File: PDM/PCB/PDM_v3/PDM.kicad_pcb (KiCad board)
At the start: 4 copper layers, 65 x 80 mm, 59 parts, among them IC1 SN74LVC1GU04DBVT, J1 12V BAT, J10 RASPBERRY PI, J11 EMU, J12 Conn_01x02_Male, J13 SAFETY SYSTEM, J16 GND, J2 EMU PIN 21 GN(AUX1), J3 EMU PIN 13 GN (AUX2), J4 BACK LIGHT, J5 COILS, J6 INJECTORS, J7 LSU 4.9, J8 RACE TCS, J9 STM BOX, U1 BTS50010-1TAE, U2 BTS50010-1TAE, U3 BTS50010-1TAE, U4 LM2937xMP

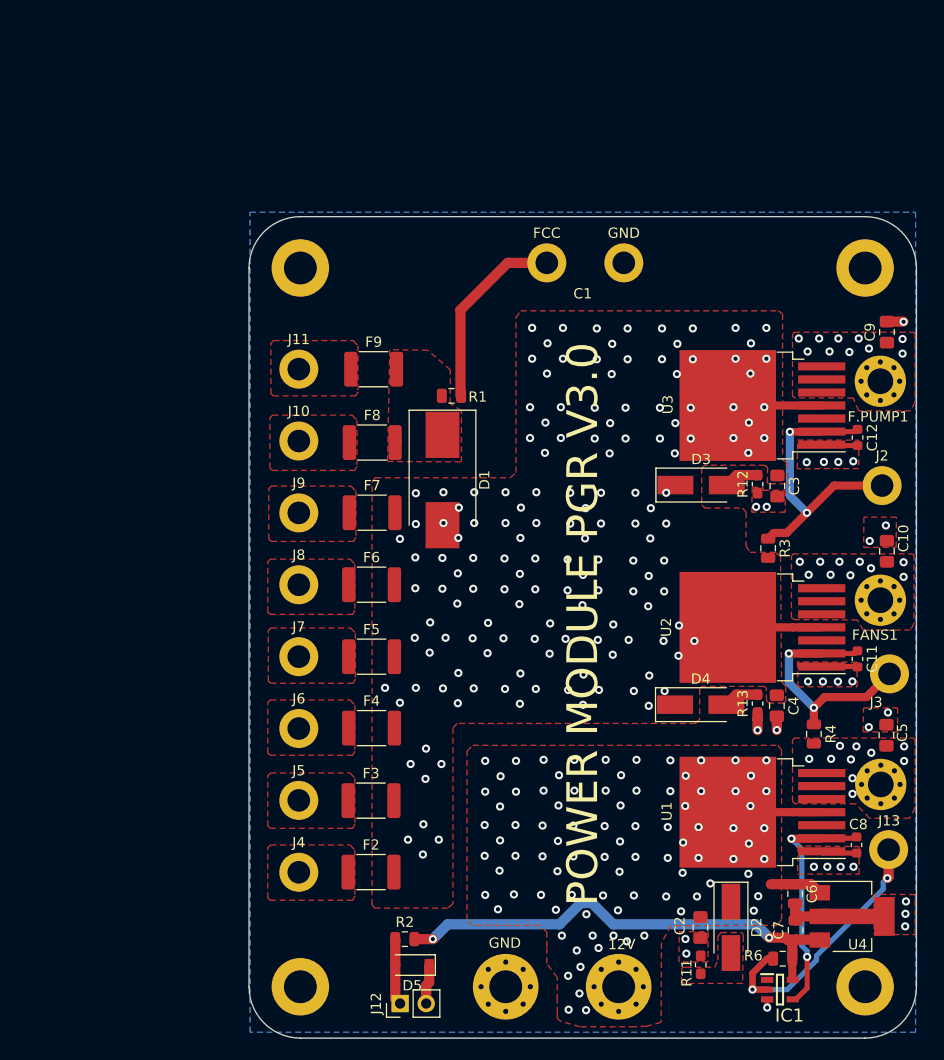
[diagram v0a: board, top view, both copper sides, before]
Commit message: Update PDM PCB
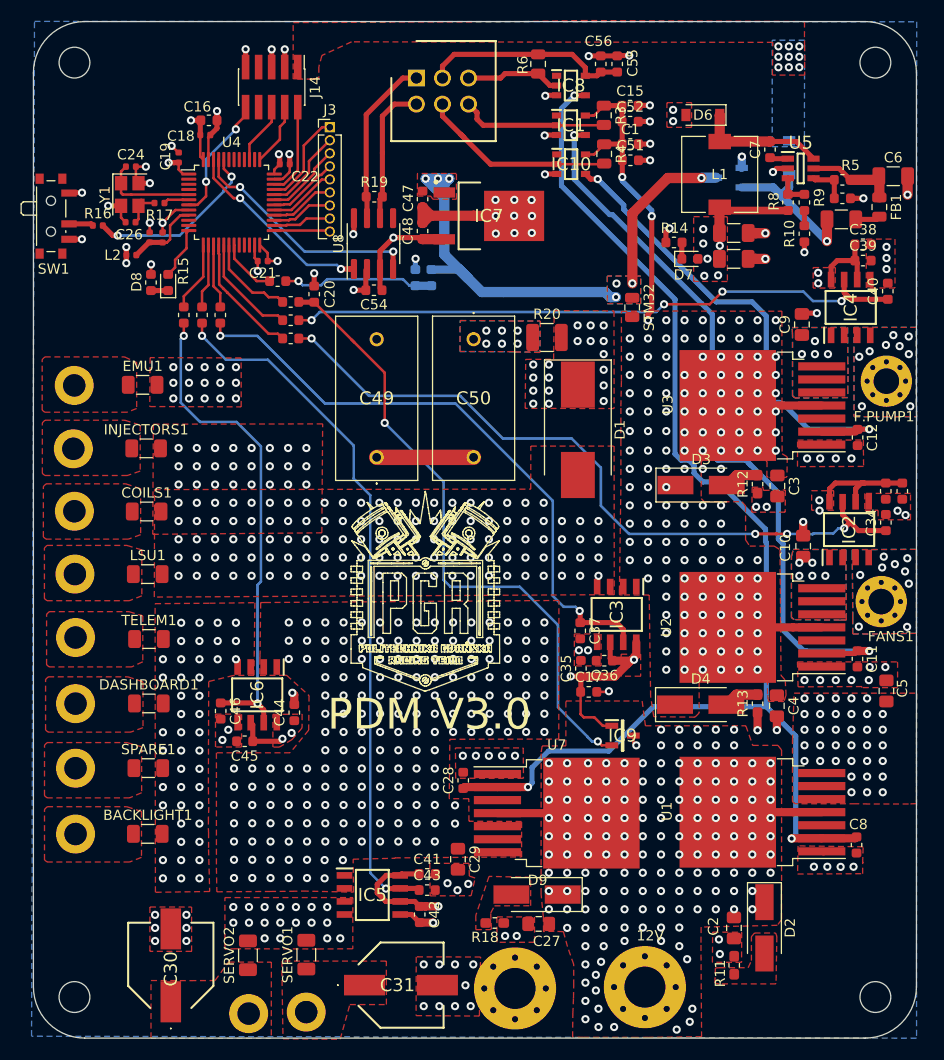
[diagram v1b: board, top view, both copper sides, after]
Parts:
- removed 12V1: 85 K1 (starter), MountingHole:MountingHole_2.5mm_Pad_Via
- removed D5: D_Schottky, Diode_SMD:D_SOD-123
- removed J12: Conn_01x02_Male, Connector_PinHeader_2.54mm:PinHeader_1x02_P2.54mm_Vertical
- removed J13: SAFETY SYSTEM, MountingHole:MountingHole_2.2mm_M2_DIN965_Pad
- added C13: 10uF, Capacitor_SMD:C_1206_3216Metric, F.Cu at (142.2, 44.6)
- added C14: 10uF, Capacitor_SMD:C_1206_3216Metric, F.Cu at (142.2, 47.1)
- added C15: 0.1uF, Capacitor_SMD:C_0603_1608Metric, F.Cu at (132.1, 32.2)
- added C16: 4u7, Capacitor_SMD:C_0603_1608Metric, F.Cu at (91.1, 33.6)
- added C17: 0.1uF, Capacitor_SMD:C_0603_1608Metric, F.Cu at (128.1, 89.3)
- added C18: 100n, Capacitor_SMD:C_0402_1005Metric, F.Cu at (90.7, 35.1)
- added C19: 100n, Capacitor_SMD:C_0402_1005Metric, F.Cu at (88.1, 37.2)
- added C20: 0.1uF, Capacitor_SMD:C_0603_1608Metric, F.Cu at (101.3, 50.5)
- added C21: 100n, Capacitor_SMD:C_0402_1005Metric, F.Cu at (96.3, 47.3)
- added C22: 100n, Capacitor_SMD:C_0402_1005Metric, F.Cu at (98.5, 37.9)
- added C23: 1u, Capacitor_SMD:C_0402_1005Metric, F.Cu at (85.3, 45.0)
- added C24: 12p, Capacitor_SMD:C_0402_1005Metric, F.Cu at (83.5, 38.1)
- added C25: 10n, Capacitor_SMD:C_0402_1005Metric, F.Cu at (86.6, 45.0)
- added C26: 12p, Capacitor_SMD:C_0402_1005Metric, F.Cu at (83.5, 43.5)
- added C27: 100nF, Capacitor_SMD:C_0805_2012Metric_Pad1.15x1.40mm_HandSolder, F.Cu at (123.2, 111.9)
- added C28: 150nF, Capacitor_SMD:C_0603_1608Metric, F.Cu at (115.9, 97.9)
- added C29: 10nF, Capacitor_SMD:C_0805_2012Metric_Pad1.15x1.40mm_HandSolder, F.Cu at (115.3, 105.6)
- added C30: 100uF, EEETP1C101AP:EEE0JA471UAP, F.Cu at (87.4, 115.9)
- added C31: 100uF, EEETP1C101AP:EEE0JA471UAP, F.Cu at (109.8, 117.8)
- added C32: 47nF, Capacitor_SMD:C_0603_1608Metric, F.Cu at (157.0, 69.7)
- added C33: 47nF, Capacitor_SMD:C_0603_1608Metric, F.Cu at (158.6, 69.7)
- added C34: 4.7nF, Capacitor_SMD:C_0603_1608Metric, F.Cu at (157.0, 72.8)
- added C35: 47nF, Capacitor_SMD:C_0603_1608Metric, F.Cu at (127.3, 87.0)
- added C36: 47nF, Capacitor_SMD:C_0603_1608Metric, F.Cu at (129.6, 86.2)
- added C37: 4.7nF, Capacitor_SMD:C_0603_1608Metric, F.Cu at (127.3, 83.3)
- added C38: 47nF, Capacitor_SMD:C_0603_1608Metric, F.Cu at (154.8, 45.7)
- added C39: 47nF, Capacitor_SMD:C_0603_1608Metric, F.Cu at (154.8, 47.3)
- added C40: 4.7nF, Capacitor_SMD:C_0603_1608Metric, F.Cu at (157.2, 50.3)
- added C41: 47nF, Capacitor_SMD:C_0603_1608Metric, F.Cu at (112.4, 107.0)
- added C42: 47nF, Capacitor_SMD:C_0603_1608Metric, F.Cu at (111.6, 111.0)
- added C43: 4.7nF, Capacitor_SMD:C_0603_1608Metric, F.Cu at (112.4, 108.6)
- added C44: 47nF, Capacitor_SMD:C_0603_1608Metric, F.Cu at (99.4, 91.3)
- added C45: 47nF, Capacitor_SMD:C_0603_1608Metric, F.Cu at (94.6, 94.1)
- added C46: 4.7nF, Capacitor_SMD:C_0603_1608Metric, F.Cu at (92.2, 91.1)
- added C47: 0.47uF, Capacitor_SMD:C_0603_1608Metric, F.Cu at (111.9, 41.3)
- added C48: 22uF, Capacitor_SMD:C_0603_1608Metric, F.Cu at (111.9, 44.4)
- added C49: SCMR18H105PRBB0, SCMR18H105PRBB0:SCMR18H105PRBB0, F.Cu at (107.4, 66.4)
- added C50: SCMR18H105PRBB0, SCMR18H105PRBB0:SCMR18H105PRBB0, F.Cu at (116.9, 54.9)
- added C51: 1uF, Capacitor_SMD:C_0603_1608Metric, F.Cu at (132.1, 37.5)
- added C52: 1uF, Capacitor_SMD:C_0603_1608Metric, F.Cu at (132.1, 33.8)
- added C54: 0.47uF, Capacitor_SMD:C_0603_1608Metric, F.Cu at (107.2, 50.2)
- added C55: 0.1uF, Capacitor_SMD:C_0603_1608Metric, F.Cu at (130.9, 28.1)
- added C56: 1uF, Capacitor_SMD:C_0603_1608Metric, F.Cu at (129.3, 28.1)
- added D11: B5819W, Diode_SMD:D_SOD-123, B.Cu at (147.6, 37.3)
- added D6: B5819W, Diode_SMD:D_SOD-123, F.Cu at (139.2, 33.1)
- added D7: LED, LED_SMD:LED_0603_1608Metric, F.Cu at (137.9, 47.1)
- added D8: BLUE, LED_SMD:LED_0603_1608Metric, F.Cu at (87.1, 49.4)
- added D9: D_TVS_ALT, Diode_SMD:D_SMA_Handsoldering, F.Cu at (123.0, 109.0)
- added F1: Polyfuse_Small, Fuse:Fuse_1206_3216Metric, F.Cu at (152.7, 43.3)
- added FB1: 600 @ 600Mhz, Inductor_SMD:L_0805_2012Metric, F.Cu at (156.4, 42.1)
- added IC10: BU4S584G2-TR, BU4S584G2-TR:SOT95P280X125-5N, F.Cu at (126.4, 37.9)
- added IC2: MLX91221KDC-ABR-020-SP, MLX91221KDC-ABR-020-SP:SOIC127P600X173-8N, F.Cu at (153.4, 73.5)
- added IC3: MLX91221KDC-ABR-020-SP, MLX91221KDC-ABR-020-SP:SOIC127P600X173-8N, F.Cu at (130.8, 81.7)
- added IC4: MLX91221KDC-ABR-020-SP, MLX91221KDC-ABR-020-SP:SOIC127P600X173-8N, F.Cu at (153.6, 51.8)
- added IC5: MLX91221KDC-ABR-020-SP, MLX91221KDC-ABR-020-SP:SOIC127P600X173-8N, F.Cu at (107.0, 109.1)
- added IC6: MLX91221KDC-ABR-020-SP, MLX91221KDC-ABR-020-SP:SOIC127P600X173-8N, F.Cu at (95.8, 89.6)
- added IC7: KF50BDT-TR, KF50BDT-TR:TO228P972X240-3N, F.Cu at (118.4, 42.9)
- added IC8: BU4S584G2-TR, BU4S584G2-TR:SOT95P280X125-5N, F.Cu at (126.4, 30.2)
- added IC9: TMP236A4DBZT, TMP236A4DBZT:SOT95P237X112-3N, F.Cu at (131.4, 93.5)
- added J14: SWD, Connector_PinHeader_1.27mm:PinHeader_2x05_P1.27mm_Vertical_SMD, F.Cu at (97.2, 30.4)
- added J15: SERVO_GEAR, MountingHole:MountingHole_2.2mm_M2_DIN965_Pad, F.Cu at (100.6, 120.5)
- added J17: SERVO_CLUTCH, MountingHole:MountingHole_2.2mm_M2_DIN965_Pad, F.Cu at (95.0, 120.6)
- added L1: 10uH, Inductor_SMD:L_7.3x7.3_H4.5, F.Cu at (140.8, 38.9)
- added L2: 39n, Inductor_SMD:L_0402_1005Metric, F.Cu at (83.5, 46.7)
- added Q1: AO3401A, AO3401A:SOT95P280X125-3N, B.Cu at (141.7, 39.2)
- added R10: 270, Resistor_SMD:R_0603_1608Metric, F.Cu at (149.1, 44.7)
- added R14: 1k, Resistor_SMD:R_0603_1608Metric, F.Cu at (136.4, 45.5)
- added R15: 1k5, Resistor_SMD:R_0603_1608Metric, F.Cu at (85.4, 49.4)
- added R16: 10k, Resistor_SMD:R_0402_1005Metric, F.Cu at (80.3, 43.9)
- added R17: 47, Resistor_SMD:R_0402_1005Metric, F.Cu at (86.3, 41.7)
- added R18: 1R, Resistor_SMD:R_0603_1608Metric_Pad1.05x0.95mm_HandSolder, F.Cu at (118.9, 111.8)
- added R19: R_Small, Resistor_SMD:R_0603_1608Metric, F.Cu at (107.2, 41.1)
- added R20: R_Small, Resistor_SMD:R_1210_3225Metric, F.Cu at (124.0, 54.8)
- added R21: 6.8k, Resistor_SMD:R_0603_1608Metric, B.Cu at (111.2, 48.9)
- added R22: 0, Resistor_SMD:R_0603_1608Metric, F.Cu at (90.4, 52.6)
- added R23: 0, Resistor_SMD:R_0603_1608Metric, F.Cu at (92.2, 52.6)
- added R24: 0, Resistor_SMD:R_0603_1608Metric, F.Cu at (99.1, 54.9)
- added R25: 0, Resistor_SMD:R_0603_1608Metric, F.Cu at (99.1, 53.1)
- added R26: 0, Resistor_SMD:R_0603_1608Metric, F.Cu at (99.1, 51.3)
- added R27: 0, Resistor_SMD:R_0603_1608Metric, F.Cu at (97.8, 49.3)
- added R5: 100k, Resistor_SMD:R_0603_1608Metric, F.Cu at (152.8, 39.4)
- added R7: 68k, Resistor_SMD:R_0603_1608Metric, F.Cu at (152.8, 41.2)
- added R8: 47k, Resistor_SMD:R_0603_1608Metric, F.Cu at (147.5, 41.6)
- added R9: 15k, Resistor_SMD:R_0603_1608Metric, F.Cu at (149.1, 41.6)
- added SERVO1: 15, Fuse:Fuse_1206_3216Metric, F.Cu at (100.6, 114.9)
- added SERVO2: 15, Fuse:Fuse_1206_3216Metric, F.Cu at (94.9, 114.9)
- added STM32: 2, Fuse:Fuse_0805_2012Metric, F.Cu at (132.3, 51.8)
- added SW1: SW_SPDT, Button_Switch_SMD:SW_SPDT_PCM12, F.Cu at (76.0, 43.0)
- added U5: MP2359, MP2359DT-LF-P:SOT95P280X145-6N, F.Cu at (148.7, 38.3)
- added U7: BTS50010-1TAE, Package_TO_SOT_SMD:TO-263-7_TabPin4, F.Cu at (125.0, 101.1)
- added U8: MCP2561-E-SN, Package_SO:SOIC-8_3.9x4.9mm_P1.27mm, F.Cu at (107.1, 45.6)
- added Y1: 8MHz, Crystal:Crystal_SMD_3225-4Pin_3.2x2.5mm, F.Cu at (83.4, 40.8)
- BACKLIGHT1: renamed from F2; footprint Fuse:Fuse_1812_4532Metric_Pad1.30x3.40mm_HandSolder -> Fuse:Fuse_1206_3216Metric
- C1: value 0.2F -> 0.1uF; footprint Kondensator:Kondensator -> Capacitor_SMD:C_0603_1608Metric
- C6: value 0.1uF -> 10uF; footprint Capacitor_SMD:C_0805_2012Metric -> Capacitor_SMD:C_1206_3216Metric
- C7: value 10uF -> 10nF; footprint Capacitor_SMD:C_0805_2012Metric -> Capacitor_SMD:C_0603_1608Metric
- COILS1: renamed from F3; footprint Fuse:Fuse_1812_4532Metric_Pad1.30x3.40mm_HandSolder -> Fuse:Fuse_1206_3216Metric
- DASHBOARD1: renamed from F7; footprint Fuse:Fuse_1812_4532Metric_Pad1.30x3.40mm_HandSolder -> Fuse:Fuse_1206_3216Metric
- EMU1: renamed from F9; footprint Fuse:Fuse_1812_4532Metric_Pad1.30x3.40mm_HandSolder -> Fuse:Fuse_1206_3216Metric
- H1, H2, H3, H4: footprint MountingHole:MountingHole_3.2mm_M3_DIN965_Pad -> MountingHole:MountingHole_3mm
- IC1: value SN74LVC1GU04DBVT -> BU4S584G2-TR; footprint SN74LVC1GU04DBVT:SOT95P280X145-5N -> BU4S584G2-TR:SOT95P280X125-5N
- INJECTORS1: renamed from F4; footprint Fuse:Fuse_1812_4532Metric_Pad1.30x3.40mm_HandSolder -> Fuse:Fuse_1206_3216Metric
- J1, J16: footprint MountingHole:MountingHole_3.2mm_M3_Pad_Via -> MountingHole:MountingHole_4mm_Pad_Via
- J10: value RASPBERRY PI -> TELEM
- J2: value EMU PIN 21 GN(AUX1) -> 90130-1106; footprint MountingHole:MountingHole_2.2mm_M2_DIN965_Pad -> 90130-1106:SHDR6W65P254_2X3_996X975X1110P
- J3: value EMU PIN 13 GN (AUX2) -> Conn_01x09_Male; footprint MountingHole:MountingHole_2.2mm_M2_DIN965_Pad -> Connector_PinHeader_1.27mm:PinHeader_1x09_P1.27mm_Vertical
- J4: value BACK LIGHT -> BACKLIGHT
- J9: value STM BOX -> DASHBOARD
- LSU1: renamed from F5; footprint Fuse:Fuse_1812_4532Metric_Pad1.30x3.40mm_HandSolder -> Fuse:Fuse_1206_3216Metric
- R1: value 0.1 -> 22k; footprint Resistor_SMD:R_0805_2012Metric -> Resistor_SMD:R_0603_1608Metric; moved to B.Cu
- R2: value 100 -> 0; footprint Resistor_SMD:R_0805_2012Metric -> Resistor_SMD:R_0603_1608Metric
- R3, R4: value 10k -> 100k
- R6: value 100 -> 100k
- SPARE1: renamed from F6; footprint Fuse:Fuse_1812_4532Metric_Pad1.30x3.40mm_HandSolder -> Fuse:Fuse_1206_3216Metric
- TELEM1: renamed from F8; footprint Fuse:Fuse_1812_4532Metric_Pad1.30x3.40mm_HandSolder -> Fuse:Fuse_1206_3216Metric
- U4: value LM2937xMP -> STM32F103C8Tx; footprint Package_TO_SOT_SMD:SOT-223-3_TabPin2 -> Package_QFP:LQFP-48_7x7mm_P0.5mm
- moved U4 92.1 mm to (93.3, 41.6)
- moved R6 90.3 mm to (123.2, 28.1), turned to 270 degrees
- moved IC1 86.6 mm to (126.3, 34.1)
- moved J3 76.2 mm to (102.9, 34.3)
- moved C7 76.1 mm to (145.7, 36.5)
- moved C6 70.5 mm to (157.7, 39.1), turned to 0 degrees
- moved R2 64.5 mm to (88.6, 52.6), turned to 90 degrees
- moved J2 60.3 mm to (111.3, 29.5)
- moved R4 60.1 mm to (129.6, 36.9)
- moved R3 45.1 mm to (129.6, 33.1)
- moved COILS1 35.6 mm to (85.0, 71.7)
- moved J5 35.6 mm to (78.0, 71.7)
- moved INJECTORS1 35.0 mm to (85.0, 65.6)
- moved J6 35.0 mm to (77.9, 65.6)
- moved H1 29.7 mm to (78.0, 28.0)
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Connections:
- BACKLIGHT1 pad 2: 12V_OUT1 -> 12V_SYSTEMS_OUT
- C1 pad 1: Net-(C1-Pad1) -> 12V_MAIN_IN
- C10 pad 1: Net-(C10-Pad1) -> FANS_MOS_IN
- C11 pad 1: IN_2 -> IN_FAN
- C12 pad 1: IN_3 -> IN_FUEL
- C3 pad 1: 12V_OUT1 -> 12V_MAIN_IN
- C4 pad 1: 12V_OUT1 -> 12V_MAIN_IN
- C5 pad 1: 12V_OUT1 -> 12V_MAIN_IN
- C6 pad 1: 12V_BAT -> BUCK_IN
- C7 pad 1: +3V3 -> BUCK_BST
- C7 pad 2: GND -> BUCK_SW
- C8 pad 1: IN_1 -> IN_MAIN_12V
- C9 pad 1: Net-(C9-Pad1) -> FUEL_MOS_IN
- COILS1 pad 2: 12V_OUT1 -> 12V_MAIN_OUT
- D1 pad 2: 12V_OUT1 -> 12V_MAIN_OUT
- D3 pad 1: 12V_OUT1 -> 12V_MAIN_IN
- D4 pad 1: 12V_OUT1 -> 12V_MAIN_IN
- DASHBOARD1 pad 2: 12V_OUT1 -> 12V_SYSTEMS_OUT
- F.PUMP1 pad 1: Net-(C9-Pad1) -> FUEL_MOS_OUT
- FANS1 pad 1: Net-(C10-Pad1) -> FANS_MOS_OUT
- IC1 pad 2: Net-(IC1-Pad2) -> EMU_AUX2
- IC1 pad 4: IN_1 -> IN_FAN
- IC1 pad 5: +3V3 -> 12V_MAIN_IN
- INJECTORS1 pad 2: 12V_OUT1 -> 12V_MAIN_OUT
- J2 pad 1: IN_3 -> CAN_H
- J3 pad 1: IN_2 -> /STM32F103C8T6/PA12
- LSU1 pad 2: 12V_OUT1 -> 12V_MAIN_OUT
- R1 pad 1: Net-(D1-Pad1) -> VOLTAGE_SENS
- R1 pad 2: Net-(C1-Pad1) -> 12V_STM32
- R2 pad 1: BSPD_IN -> CURRENT_12V_SYSTEMS
- R2 pad 2: +3V3 -> /STM32F103C8T6/PA3
- R3 pad 1: IN_3 -> 12V_MAIN_IN
- R3 pad 2: 12V_OUT1 -> EMU_AUX2
- R4 pad 1: IN_2 -> 12V_MAIN_IN
- R4 pad 2: 12V_OUT1 -> EMU_AUX1
- R6 pad 1: +3V3 -> 12V_BAT
- R6 pad 2: Net-(IC1-Pad2) -> SAFETY_LINE
- SPARE1 pad 2: 12V_OUT1 -> 12V_SYSTEMS_OUT
- TELEM1 pad 2: Net-(D1-Pad1) -> 12V_SYSTEMS_OUT
- U1 pad 2: IN_1 -> IN_MAIN_12V
- U1 pad 5: 12V_OUT1 -> 12V_MAIN_IN
- U1 pad 6: 12V_OUT1 -> 12V_MAIN_IN
- U1 pad 7: 12V_OUT1 -> 12V_MAIN_IN
- U2 pad 2: IN_2 -> IN_FAN
- U2 pad 4: 12V_OUT1 -> 12V_MAIN_IN
- U2 pad 5: Net-(C10-Pad1) -> FANS_MOS_IN
- U2 pad 6: Net-(C10-Pad1) -> FANS_MOS_IN
- U2 pad 7: Net-(C10-Pad1) -> FANS_MOS_IN
- U3 pad 2: IN_3 -> IN_FUEL
- U3 pad 4: 12V_OUT1 -> 12V_MAIN_IN
- U3 pad 5: Net-(C9-Pad1) -> FUEL_MOS_IN
- U3 pad 6: Net-(C9-Pad1) -> FUEL_MOS_IN
- U3 pad 7: Net-(C9-Pad1) -> FUEL_MOS_IN
- U4 pad 1: 12V_BAT -> +3V3
- U4 pad 2: GND -> (no net)
- U4 pad 3: +3V3 -> (no net)
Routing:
- net +3V3: track 46.4 -> 248.2 mm, vias 2 -> 22
- net IN_MAIN_12V: track 0.00 -> 125.0 mm, vias 0 -> 3
- net IN_FAN: track 0.00 -> 73.8 mm, vias 0 -> 2
- net CURRENT_FANS: track 0.00 -> 72.7 mm, vias 0 -> 4
- net CURRENT_SERVO: track 0.00 -> 68.3 mm, vias 0 -> 2
- net TEMP: track 0.00 -> 61.9 mm, vias 0 -> 2
- net GND: track 27.4 -> 89.2 mm, vias 27 -> 107
- net CURRENT_FUEL: track 0.00 -> 61.3 mm, vias 0 -> 4
- net CURRENT_12V_MAIN: track 0.00 -> 59.6 mm, vias 0 -> 2
- net 12V_STM32: track 0.00 -> 52.9 mm, vias 0 -> 7
- net 12V_MAIN_IN: track 0.00 -> 48.5 mm, vias 0 -> 176
- net CURRENT_12V_SYSTEMS: track 0.00 -> 48.4 mm, vias 0 -> 2
- net IN_FUEL: track 0.00 -> 47.6 mm, vias 0 -> 2
- net IN_3: track 28.5 -> 0.00 mm, vias 2 -> 0
- net Net-(IC1-Pad2): track 26.7 -> 0.00 mm, vias 2 -> 0
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- added copper zone on F.Cu, net +3V3
- added copper zone on In2.Cu, net +3V3
- added copper zone on F.Cu, net 12V_MAIN_IN
- added copper zone on In1.Cu, net 12V_MAIN_IN
- added copper zone on F.Cu, net 12V_MAIN_OUT
- added copper zone on In1.Cu, net 12V_MAIN_OUT
- added copper zone on F.Cu, net 12V_SERVO_OUT
- added copper zone on In1.Cu, net 12V_SERVO_OUT
- added copper zone on B.Cu, net 12V_STM32
- added copper zone on F.Cu, net 12V_STM32
- added copper zone on F.Cu, net 12V_SYSTEMS
- added copper zone on In1.Cu, net 12V_SYSTEMS
- added copper zone on F.Cu, net 12V_SYSTEMS_OUT
- added copper zone on In1.Cu, net 12V_SYSTEMS_OUT
- added copper zone on B.Cu, net 5V_ST_LINK
- added copper zone on F.Cu, net 5V_ST_LINK
- added copper zone on B.Cu, net FANS_MOS_IN
- added copper zone on F.Cu, net FANS_MOS_IN
- added copper zone on B.Cu, net FANS_MOS_OUT
- added copper zone on F.Cu, net FANS_MOS_OUT
- added copper zone on B.Cu, net FUEL_MOS_IN
- added copper zone on F.Cu, net FUEL_MOS_IN
- added copper zone on B.Cu, net FUEL_MOS_OUT
- added copper zone on F.Cu, net FUEL_MOS_OUT
- added copper zone on F.Cu, net Net-(C30-Pad1)
- added copper zone on F.Cu, net Net-(C31-Pad1)
- added copper zone on B.Cu, net Net-(C50-Pad1)
- added copper zone on F.Cu, net Net-(C50-Pad1)
- added copper zone on In2.Cu, net Net-(D1-Pad1)
- added copper zone on F.Cu, net Net-(D9-Pad2)
- removed copper zone on F.Cu, net 12V_OUT1
- removed copper zone on In1.Cu, net 12V_OUT1
- removed copper zone on F.Cu, net Net-(C10-Pad1)
- removed copper zone on F.Cu, net Net-(C9-Pad1)
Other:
- board size 65 x 80 mm -> 86 x 99 mm
- board text added: "PDM V3.0"
- board text removed: "POWER MODULE PGR V3.0"
